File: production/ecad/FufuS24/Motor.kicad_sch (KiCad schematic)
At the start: 12 parts, among them J10 Conn_01x02, J11 Conn_01x02, J12 Conn_01x02, J13 Conn_01x03_Socket, J5 Conn_01x02, J6 Conn_01x02, J7 Conn_01x03_Socket, J8 Conn_01x02, J9 Conn_01x02

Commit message: efan 3
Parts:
- J5, J6, J7: footprint (none) -> footprints:CONN2_710002_WRE
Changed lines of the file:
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@@
       (effects (font (size 1.27 1.27)))
     )
-    (property "Footprint" "" (at 32.385 60.325 0)
+    (property "Footprint" "footprints:CONN2_710002_WRE" (at 32.385 60.325 0)
       (effects (font (size 1.27 1.27)) hide)
     )
@@
       (effects (font (size 1.27 1.27)))
     )
-    (property "Footprint" "" (at 31.115 83.82 0)
+    (property "Footprint" "footprints:CONN2_710002_WRE" (at 31.115 83.82 0)
       (effects (font (size 1.27 1.27)) hide)
     )
@@
       (effects (font (size 1.27 1.27)))
     )
-    (property "Footprint" "" (at 32.385 38.1 0)
-      (effects (font (size 1.27 1.27)) hide)
-    )
+    (property "Footprint" "footprints:CONN2_710002_WRE" (at 32.385 38.1 0)
+      (effects (font (size 1.27 1.27)) hide)
+    )

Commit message: efan 5
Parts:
- J10, J11, J12, J8, J9: footprint (none) -> footprints:CON_5025840270_MOL
- TP6, TP7, TP8: footprint TestPoint:TestPoint_Pad_2.0x2.0mm -> footprints:TP_5014
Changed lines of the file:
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@@
       (effects (font (size 1.27 1.27)))
     )
-    (property "Footprint" "" (at 32.385 104.775 0)
+    (property "Footprint" "footprints:CON_5025840270_MOL" (at 32.385 104.775 0)
       (effects (font (size 1.27 1.27)) hide)
     )
@@
       (effects (font (size 1.27 1.27)) (justify left))
     )
-    (property "Footprint" "TestPoint:TestPoint_Pad_2.0x2.0mm" (at 111.76 54.61 0)
+    (property "Footprint" "footprints:TP_5014" (at 111.76 54.61 0)
       (effects (font (size 1.27 1.27)) hide)
     )
@@
       (effects (font (size 1.27 1.27)))
     )
-    (property "Footprint" "" (at 32.385 151.13 0)
+    (property "Footprint" "footprints:CON_5025840270_MOL" (at 32.385 151.13 0)
       (effects (font (size 1.27 1.27)) hide)
     )
@@
       (effects (font (size 1.27 1.27)))
     )
-    (property "Footprint" "" (at 32.385 132.715 0)
+    (property "Footprint" "footprints:CON_5025840270_MOL" (at 32.385 132.715 0)
       (effects (font (size 1.27 1.27)) hide)
     )
@@
       (effects (font (size 1.27 1.27)) (justify left))
     )
-    (property "Footprint" "TestPoint:TestPoint_Pad_2.0x2.0mm" (at 109.855 43.815 0)
+    (property "Footprint" "footprints:TP_5014" (at 109.855 43.815 0)
       (effects (font (size 1.27 1.27)) hide)
     )
@@
       (effects (font (size 1.27 1.27)))
     )
-    (property "Footprint" "" (at 32.385 110.49 0)
+    (property "Footprint" "footprints:CON_5025840270_MOL" (at 32.385 110.49 0)
       (effects (font (size 1.27 1.27)) hide)
     )
@@
       (effects (font (size 1.27 1.27)) (justify right))
     )
-    (property "Footprint" "TestPoint:TestPoint_Pad_2.0x2.0mm" (at 99.695 55.88 0)
+    (property "Footprint" "footprints:TP_5014" (at 99.695 55.88 0)
       (effects (font (size 1.27 1.27)) hide)
     )
@@
       (effects (font (size 1.27 1.27)))
     )
-    (property "Footprint" "" (at 32.385 127 0)
-      (effects (font (size 1.27 1.27)) hide)
-    )
+    (property "Footprint" "footprints:CON_5025840270_MOL" (at 32.385 127 0)
+      (effects (font (size 1.27 1.27)) hide)
+    )

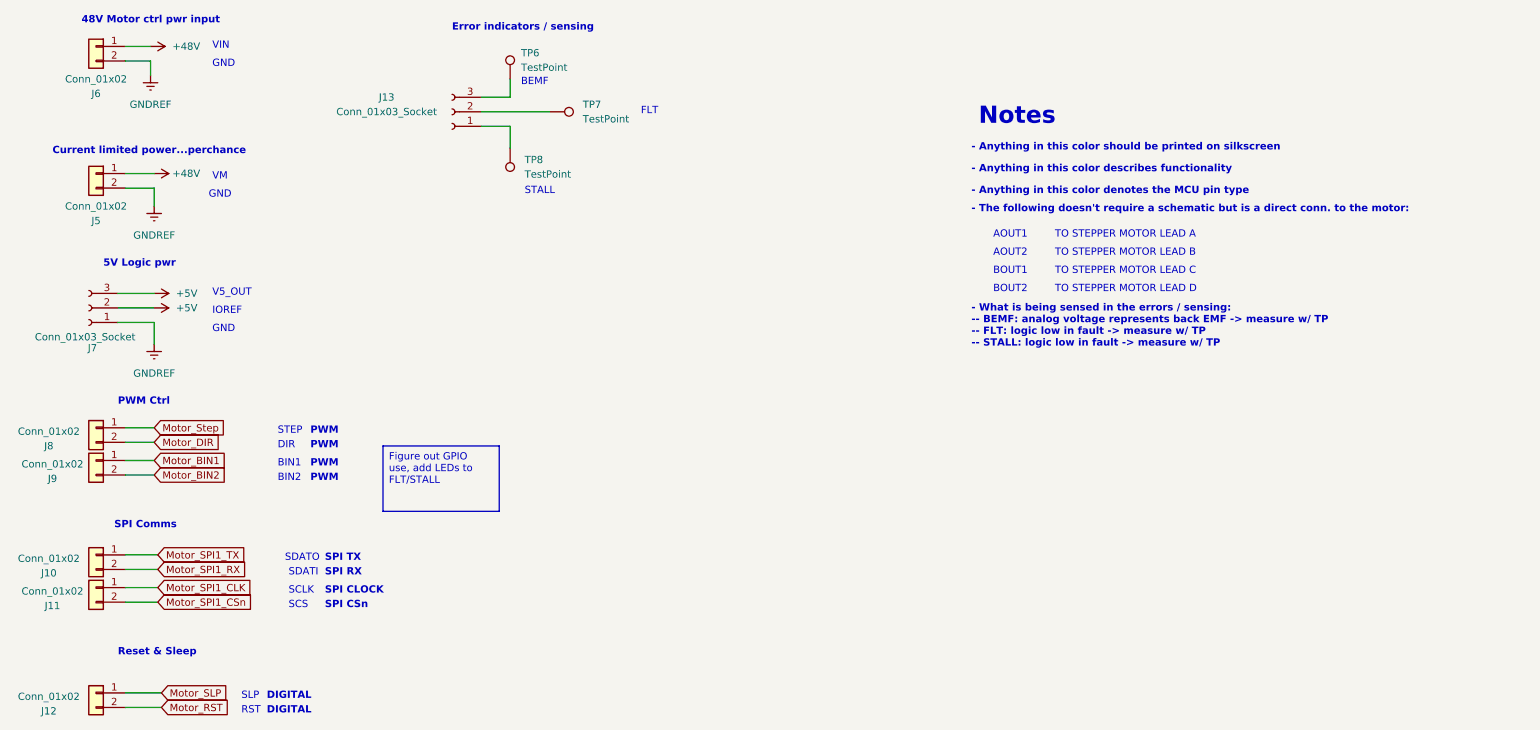
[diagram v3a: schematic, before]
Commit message: goose
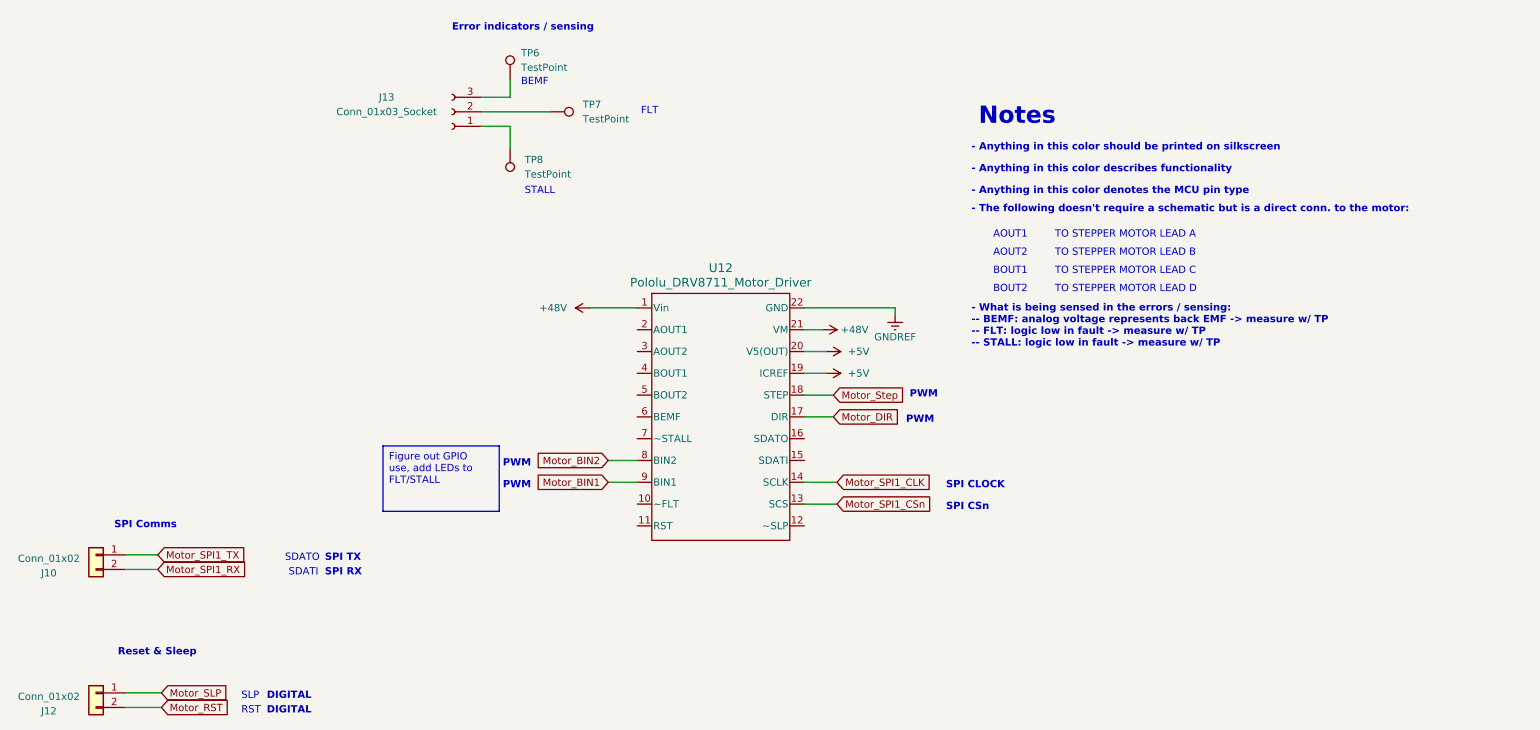
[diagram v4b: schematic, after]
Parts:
- removed J11, J8, J9: Conn_01x02, footprints:CON_5025840270_MOL, symbol Connector_Generic:Conn_01x02
- removed J5, J6: Conn_01x02, footprints:CONN2_710002_WRE, symbol Connector_Generic:Conn_01x02
- removed J7: Conn_01x03_Socket, footprints:CONN2_710002_WRE, symbol Connector:Conn_01x03_Socket
- added U12: Pololu_DRV8711_Motor_Driver, symbol POLOLU_35v4:Pololu_DRV8711_Motor_Driver
- J10, J12: footprint footprints:CON_5025840270_MOL -> (none)
- TP6, TP7, TP8: footprint footprints:TP_5014 -> TestPoint:TestPoint_Pad_2.0x2.0mm
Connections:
- net +48V: now also U12.1 (Vin), U12.21 (VM)
- net +5V: now also U12.19 (ICREF), U12.20 (V5(OUT))
- net GNDREF: now also U12.22 (GND)
- net Motor_BIN1: now also U12.9 (BIN1)
- net Motor_BIN2: now also U12.8 (BIN2)
- net Motor_DIR: now also U12.17 (DIR)
- net Motor_SPI1_CLK: now also U12.14 (SCLK)
- net Motor_SPI1_CSn: now also U12.13 (SCS)
- net Motor_Step: now also U12.18 (STEP)
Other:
- note removed: "48V Motor ctrl pwr input"
- note removed: "5V Logic pwr"
- note removed: "BIN1"
- note removed: "BIN2"
- note removed: "Current limited power...perchance"
- note removed: "DIR"
- note removed: "GND"
- note removed: "IOREF"
- note removed: "PWM Ctrl"
- note removed: "SCLK"
- note removed: "SCS"
- note removed: "STEP"
- note removed: "V5_OUT"
- note removed: "VIN"
- note removed: "VM"
